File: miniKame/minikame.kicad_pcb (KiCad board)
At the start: 2 copper layers, 48.8 x 40.1 mm, 16 parts, among them J1 PWM, J10 C, J11 A, J12 D, J13 B, J2 Camera, J3 ESP32, J4 ESP32, J5 GND, J6 Vcc, J7 UART, J8 I2C, J9 Motor

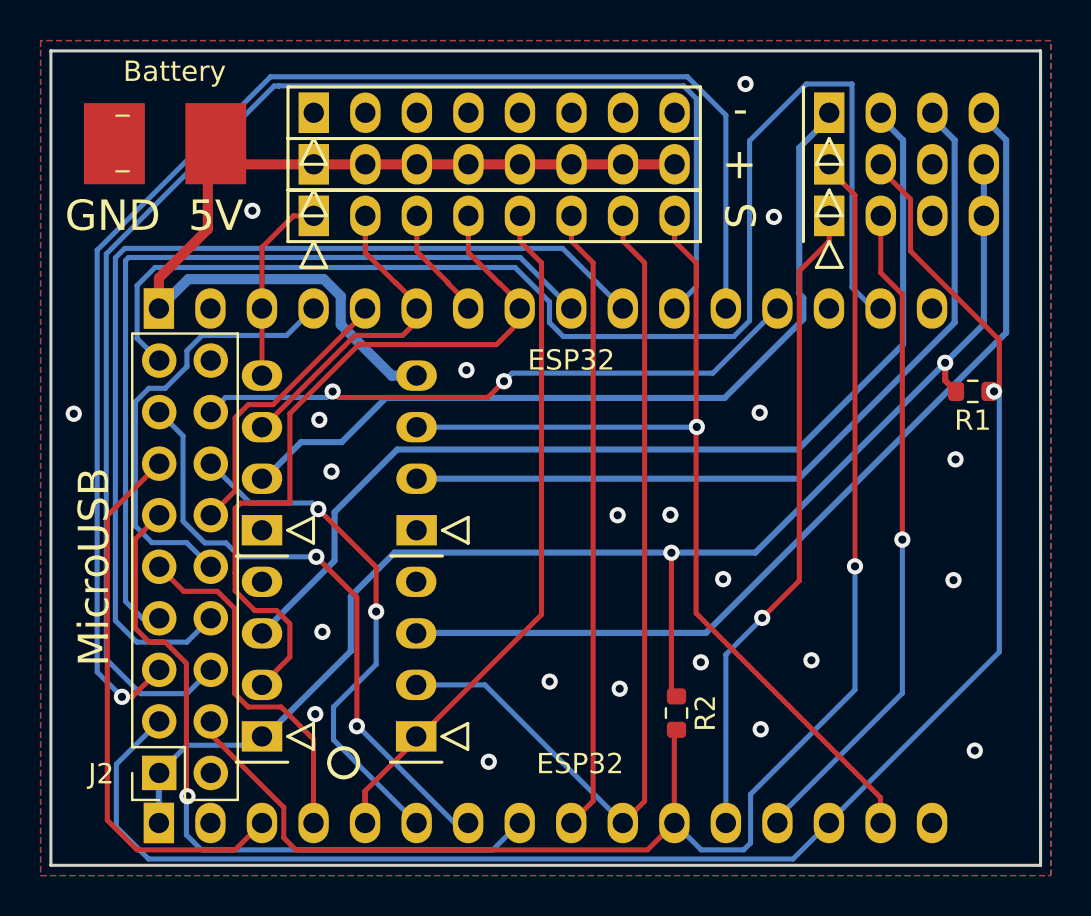
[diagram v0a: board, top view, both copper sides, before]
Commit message: save
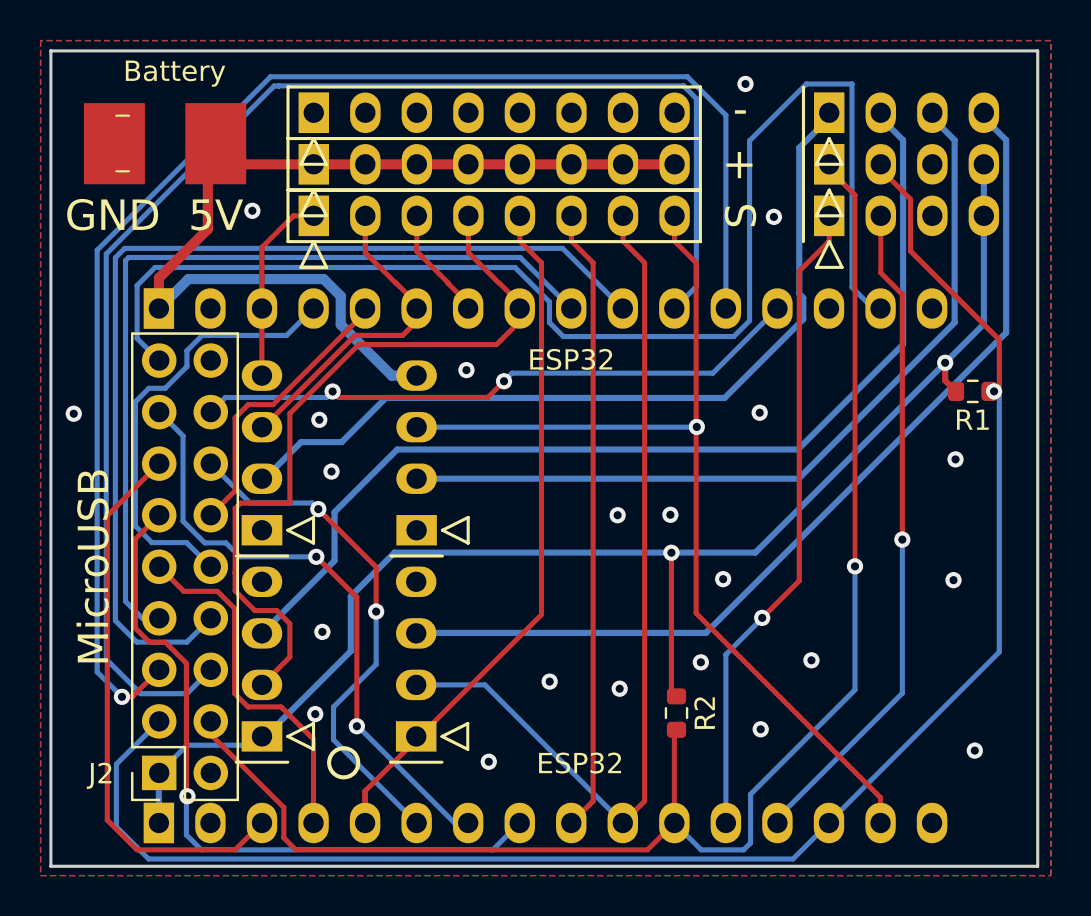
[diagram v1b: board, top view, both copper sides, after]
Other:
- board size 48.8 x 40.1 mm -> 48.6 x 40.2 mm
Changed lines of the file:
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@@
   )
   (gr_circle (center 133.3 118.9) (end 133.808 119.408) (layer "F.SilkS") (width 0.2) (fill none))
-  (gr_line (start 167.64 83.82) (end 167.64 123.952) (layer "Edge.Cuts") (width 0.15))
-  (gr_line (start 118.872 83.82) (end 167.64 83.82) (layer "Edge.Cuts") (width 0.15))
-  (gr_line (start 118.872 123.952) (end 118.872 83.82) (layer "Edge.Cuts") (width 0.15))
-  (gr_line (start 167.64 123.952) (end 118.872 123.952) (layer "Edge.Cuts") (width 0.15))
+  (gr_line (start 167.5 83.82) (end 167.5 124) (layer "Edge.Cuts") (width 0.15))
+  (gr_line (start 118.872 83.82) (end 167.5 83.82) (layer "Edge.Cuts") (width 0.15))
+  (gr_line (start 118.872 124) (end 118.872 83.82) (layer "Edge.Cuts") (width 0.15))
+  (gr_line (start 167.5 124) (end 118.872 124) (layer "Edge.Cuts") (width 0.15))
   (gr_text "v2.3" (at 141.55 106.85 90) (layer "B.SilkS")
     (effects (font (size 1.5 1.5) (thickness 0.3)) (justify mirror))
@@
   )
   (dimension (type aligned) (layer "Dwgs.User")
-    (pts (xy 167.64 123.952) (xy 167.64 83.82))
+    (pts (xy 167.5 124) (xy 167.5 83.82))
     (height 8.21)
-    (gr_text "40.1320 mm" (at 174.05 103.886 90) (layer "Dwgs.User")
+    (gr_text "40,1800 mm" (at 173.91 103.91 90) (layer "Dwgs.User")
       (effects (font (size 1.5 1.5) (thickness 0.3)))
     )
@@
   )
   (dimension (type aligned) (layer "Dwgs.User")
-    (pts (xy 167.64 83.82) (xy 118.872 83.82))
+    (pts (xy 167.5 83.82) (xy 118.872 83.82))
     (height 7.62)
-    (gr_text "48.7680 mm" (at 143.256 74.4) (layer "Dwgs.User")
+    (gr_text "48,6280 mm" (at 143.186 74.4) (layer "Dwgs.User")
       (effects (font (size 1.5 1.5) (thickness 0.3)))
     )
